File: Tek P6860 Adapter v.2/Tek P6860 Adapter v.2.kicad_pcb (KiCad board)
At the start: 2 copper layers, 36.6 x 69.3 mm, 6 parts, among them J1 Conn_01x08, J2 Conn_01x08, J3 Conn_01x02, J4 P6860_Pads, J5 Conn_01x09, SW1 SW_DIP_x09

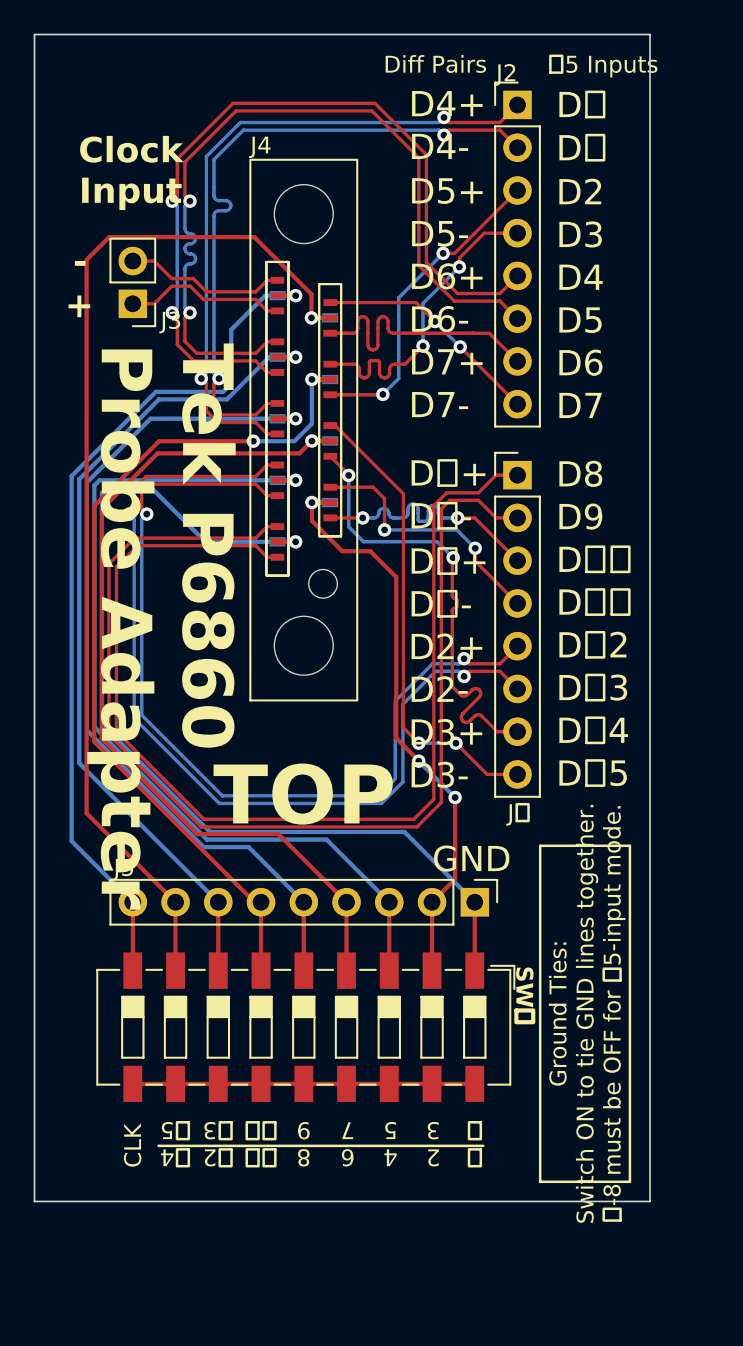
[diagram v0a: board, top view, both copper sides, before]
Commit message: Add files via upload
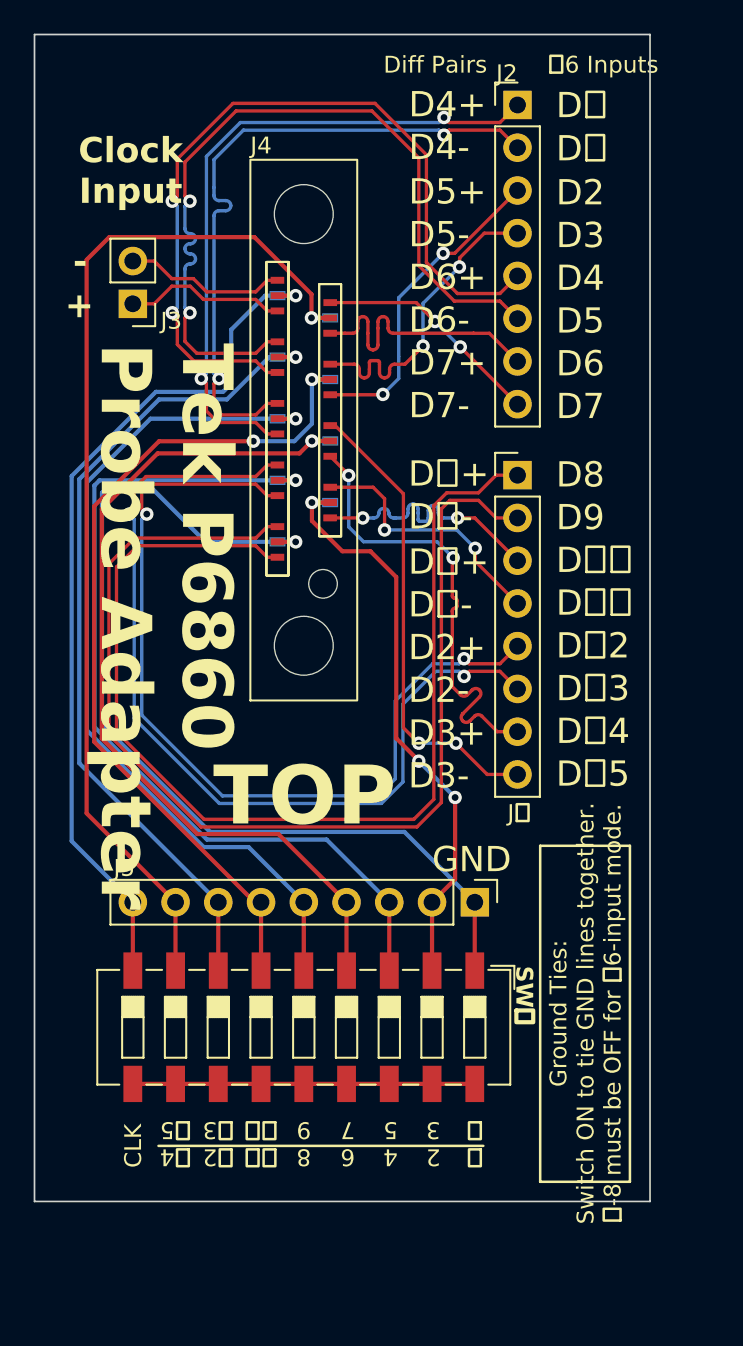
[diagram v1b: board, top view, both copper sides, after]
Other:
- board text added: "Ground Ties: Switch ON to tie GND lines together. -8 must be OFF for 6-input mode."
- board text added: "6 Inputs"
- board text removed: "Ground Ties: Switch ON to tie GND lines together. -8 must be OFF for 5-input mode."
- board text removed: "5 Inputs"
